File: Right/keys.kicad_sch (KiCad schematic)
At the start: 18 parts, among them K1 KeyboardSwitch, K10 KeyboardSwitch, K11 KeyboardSwitch, K12 KeyboardSwitch, K13 KeyboardSwitch, K14 KeyboardSwitch, K15 KeyboardSwitch, K16 KeyboardSwitch, K17 KeyboardSwitch, K18 KeyboardSwitch, K2 KeyboardSwitch, K3 KeyboardSwitch, K4 KeyboardSwitch, K5 KeyboardSwitch, K6 KeyboardSwitch, K7 KeyboardSwitch, K8 KeyboardSwitch, K9 KeyboardSwitch

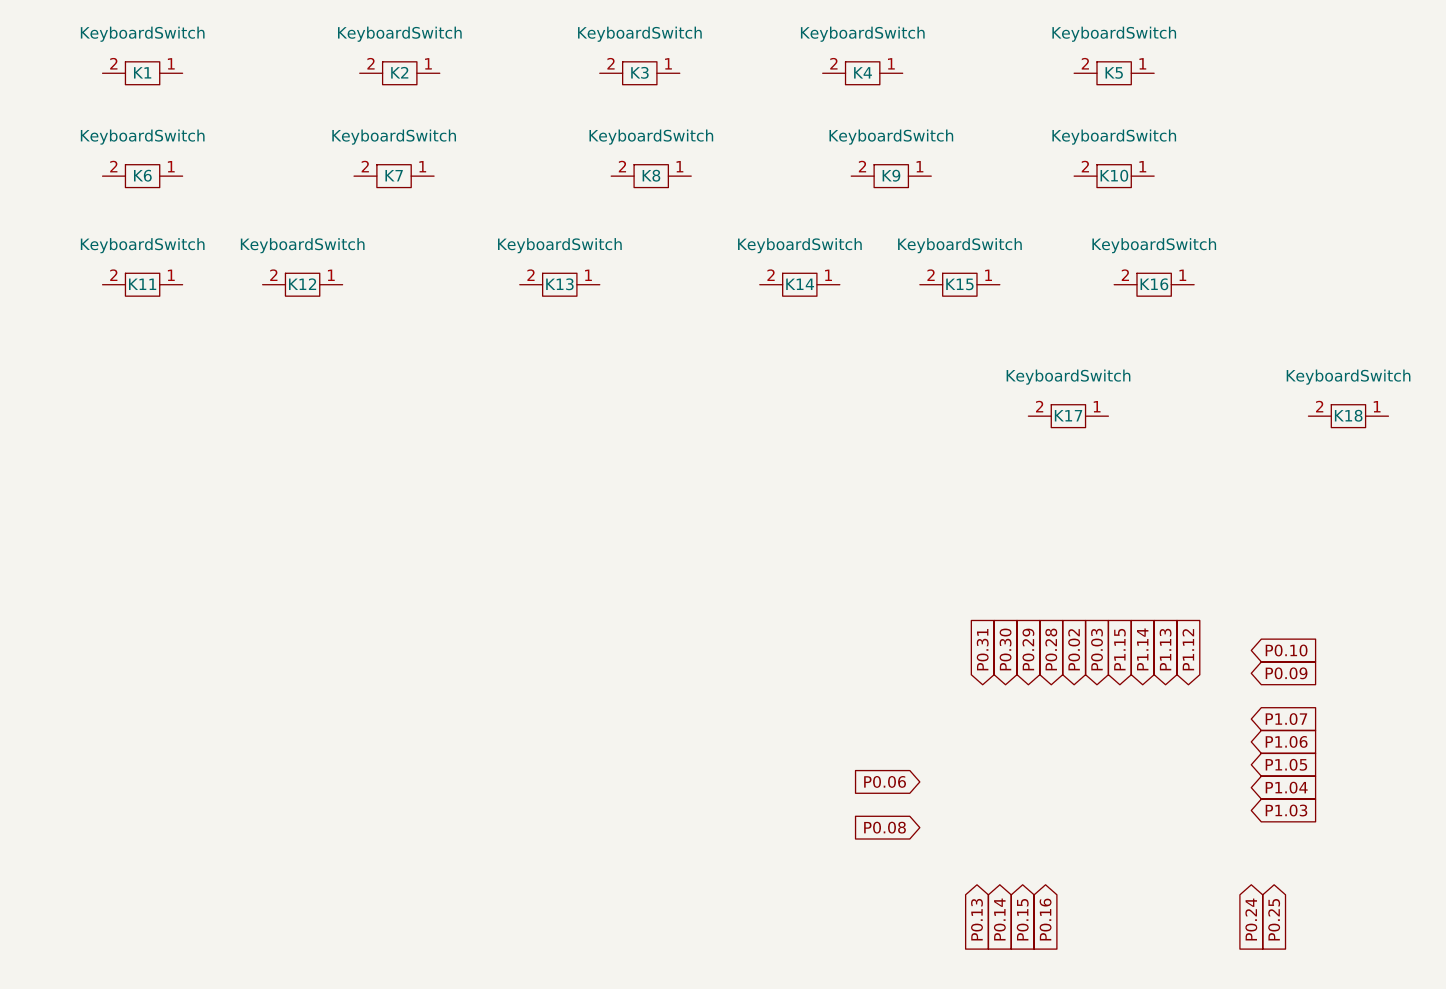
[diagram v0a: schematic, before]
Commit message: routed right hand
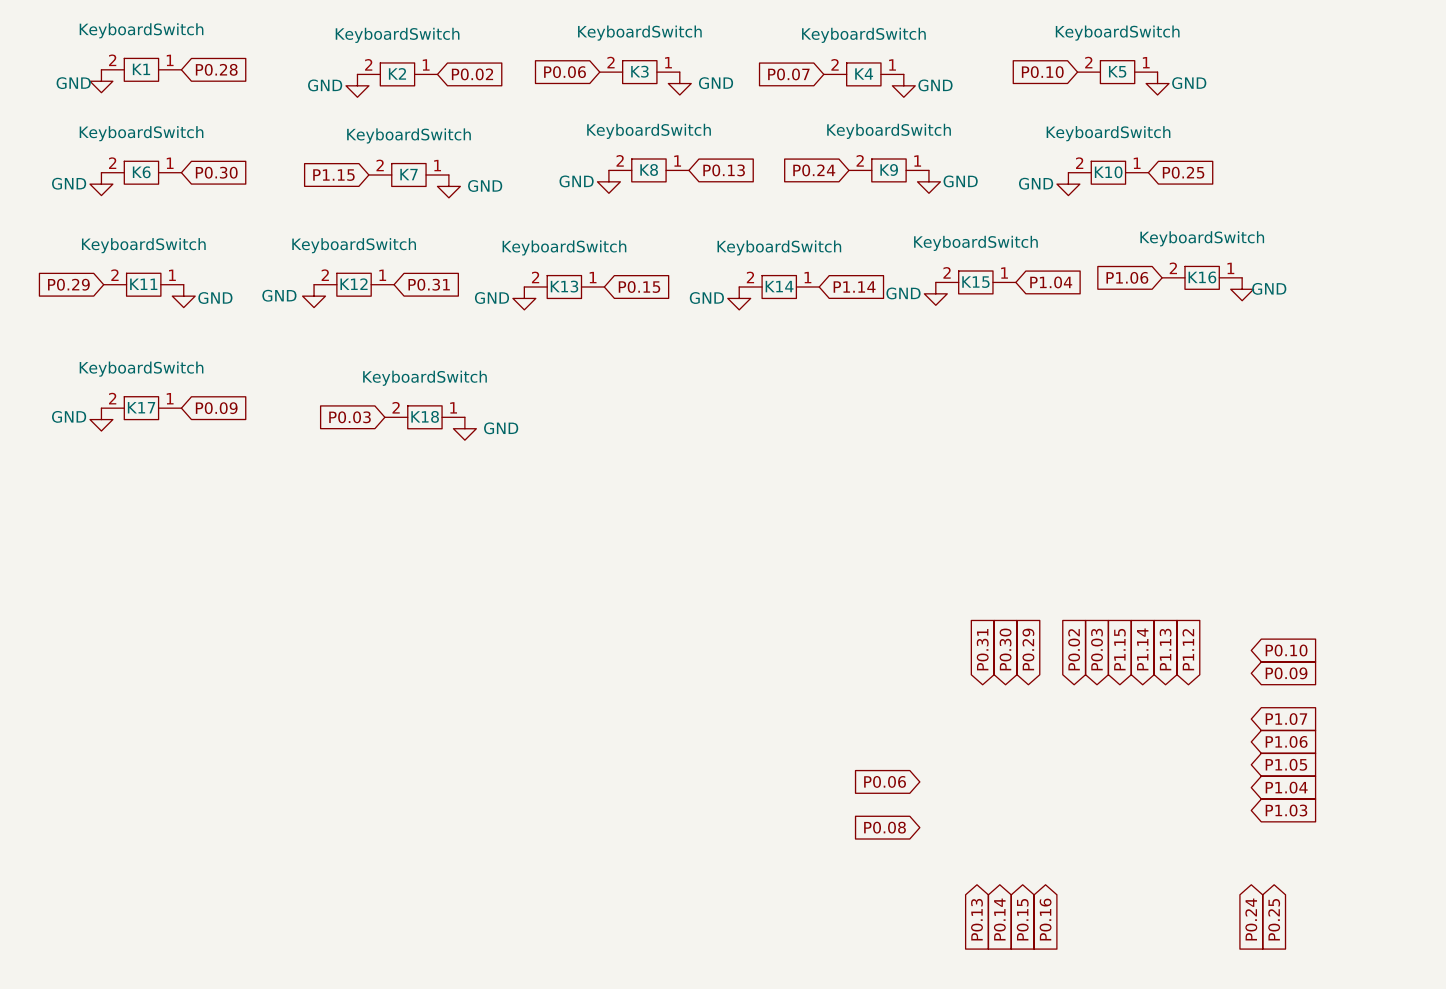
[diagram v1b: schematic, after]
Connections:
- net P0.02: now also K2.1
- net P0.03: now also K18.2
- net P0.06: now also K3.2
- net P0.09: now also K17.1
- net P0.10: now also K5.2
- net P0.13: now also K8.1
- net P0.15: now also K13.1
- net P0.24: now also K9.2
- net P0.25: now also K10.1
- net P0.28: now also K1.1
- net P0.29: now also K11.2
- net P0.30: now also K6.1
- net P0.31: now also K12.1
- net P1.04: now also K15.1
- net P1.06: now also K16.2
- net P1.14: now also K14.1
- net P1.15: now also K7.2
- net GND: now reaches K14.2
- net GND: now also K1.2, K10.2, K11.1, K12.2, K13.2, K15.2, K16.1, K17.2, K18.1, K2.2, K3.1, K4.1, K5.1, K6.2, K7.1, K8.2, K9.1
- net P0.07: now reaches K4.2
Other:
- moved on the sheet: K10, K12, K13, K14, K15, K16, K17, K18, K7, K8, K9
